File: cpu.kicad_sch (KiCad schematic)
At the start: 33 parts, among them IC12 DS2401+, IC13 ARM250, IC20 74HC138, IC27 74AC32, IC8 74HCT14, X4 72.0MHz, X5 25.175MHz

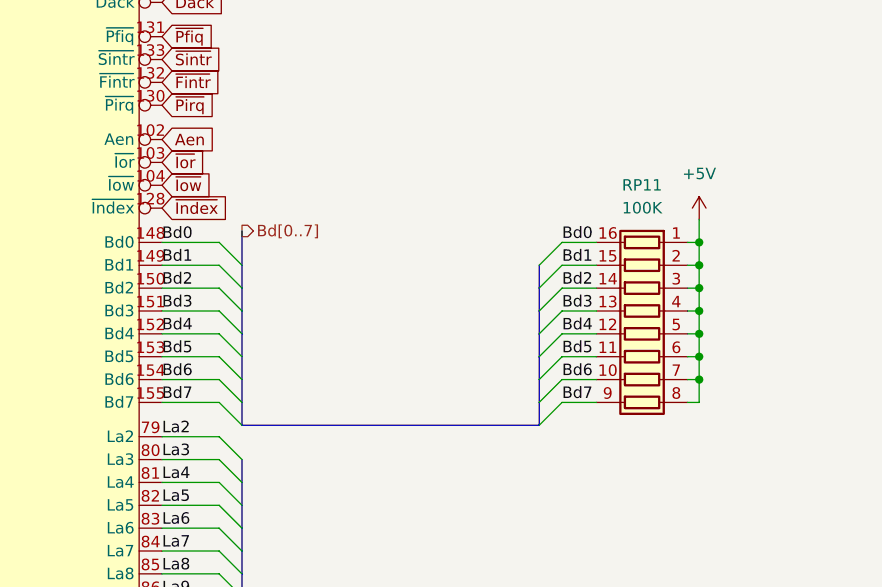
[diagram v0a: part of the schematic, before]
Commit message: fix rp11
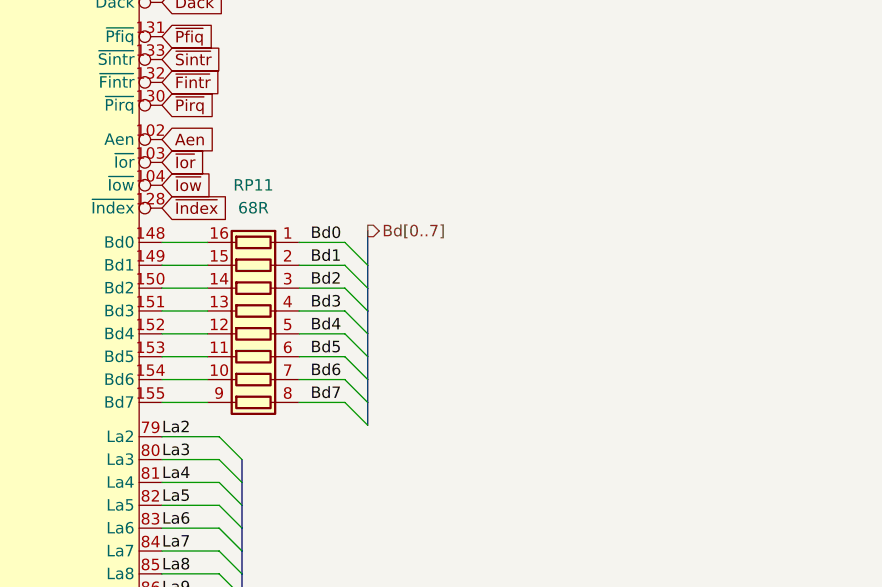
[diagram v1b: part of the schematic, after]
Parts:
- RP11: value 100K -> 68R
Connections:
- net +5V: no longer RP11.1 (R1.1), RP11.2 (R2.1), RP11.3 (R3.1), RP11.4 (R4.1), RP11.5 (R5.1), RP11.6 (R6.1), RP11.7 (R7.1), RP11.8 (R8.1)
- net Bd0: now also RP11.1 (R1.1); no longer IC13.148 (Bd0), RP11.16 (R1.2)
- net Bd1: now also RP11.2 (R2.1); no longer IC13.149 (Bd1), RP11.15 (R2.2)
- net Bd2: now also RP11.3 (R3.1); no longer IC13.150 (Bd2), RP11.14 (R3.2)
- net Bd3: now also RP11.4 (R4.1); no longer IC13.151 (Bd3), RP11.13 (R4.2)
- net Bd4: now also RP11.5 (R5.1); no longer IC13.152 (Bd4), RP11.12 (R5.2)
- net Bd5: now also RP11.6 (R6.1); no longer IC13.153 (Bd5), RP11.11 (R6.2)
- net Bd6: now also RP11.7 (R7.1); no longer IC13.154 (Bd6), RP11.10 (R7.2)
- net Bd7: now also RP11.8 (R8.1); no longer IC13.155 (Bd7), RP11.9 (R8.2)
- new net: IC13.154 (Bd6), RP11.10 (R7.2)
- new net: IC13.153 (Bd5), RP11.11 (R6.2)
- new net: IC13.152 (Bd4), RP11.12 (R5.2)
- new net: IC13.151 (Bd3), RP11.13 (R4.2)
- new net: IC13.150 (Bd2), RP11.14 (R3.2)
- new net: IC13.149 (Bd1), RP11.15 (R2.2)
- new net: IC13.148 (Bd0), RP11.16 (R1.2)
- new net: IC13.155 (Bd7), RP11.9 (R8.2)
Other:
- moved on the sheet: RP11

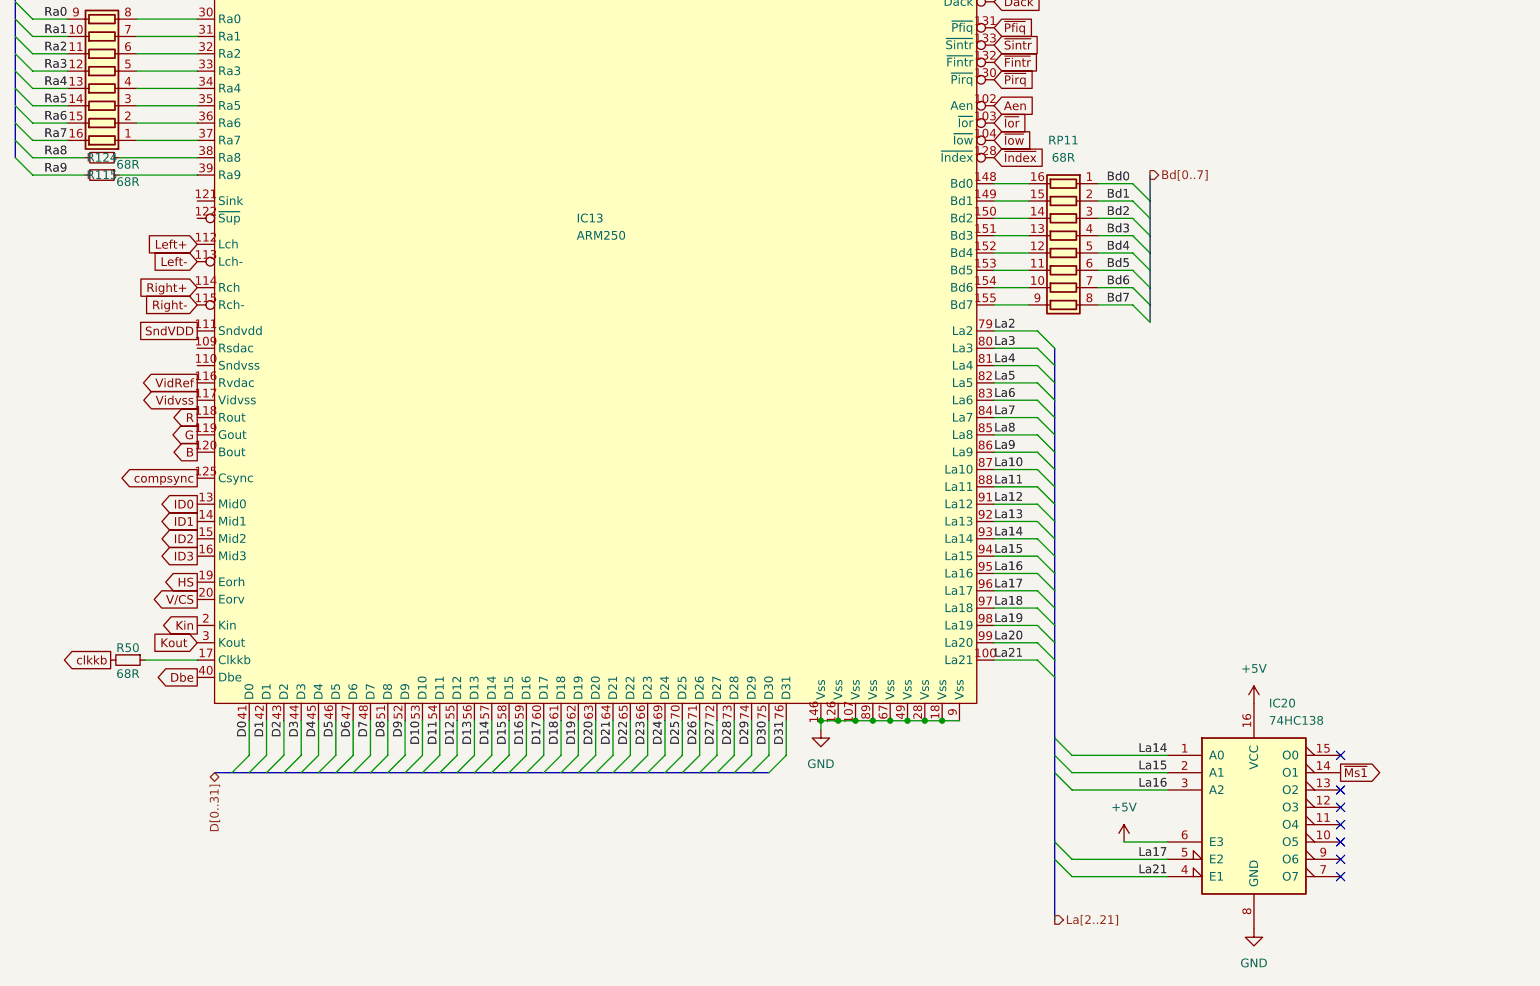
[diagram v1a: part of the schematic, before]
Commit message: more traces
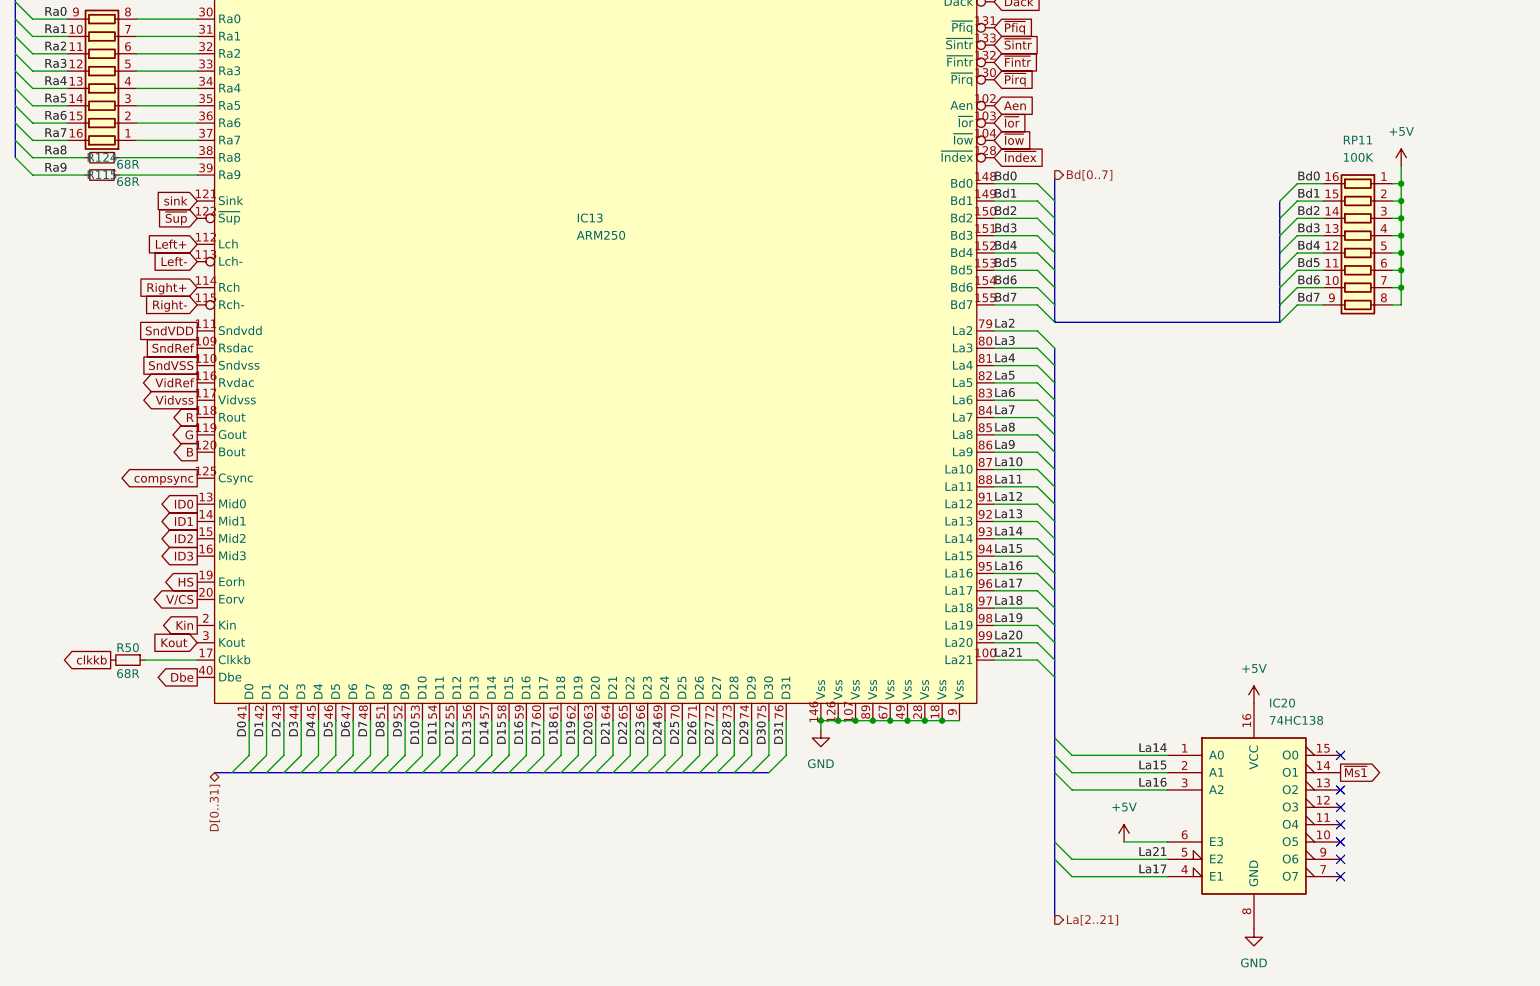
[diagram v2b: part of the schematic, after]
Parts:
- RP11: value 68R -> 100K
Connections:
- net +5V: now also RP11.1 (R1.1), RP11.2 (R2.1), RP11.3 (R3.1), RP11.4 (R4.1), RP11.5 (R5.1), RP11.6 (R6.1), RP11.7 (R7.1), RP11.8 (R8.1)
- net Bd0: now also IC13.148 (Bd0), RP11.16 (R1.2); no longer RP11.1 (R1.1)
- net Bd1: now also IC13.149 (Bd1), RP11.15 (R2.2); no longer RP11.2 (R2.1)
- net Bd2: now also IC13.150 (Bd2), RP11.14 (R3.2); no longer RP11.3 (R3.1)
- net Bd3: now also IC13.151 (Bd3), RP11.13 (R4.2); no longer RP11.4 (R4.1)
- net Bd4: now also IC13.152 (Bd4), RP11.12 (R5.2); no longer RP11.5 (R5.1)
- net Bd5: now also IC13.153 (Bd5), RP11.11 (R6.2); no longer RP11.6 (R6.1)
- net Bd6: now also IC13.154 (Bd6), RP11.10 (R7.2); no longer RP11.7 (R7.1)
- net Bd7: now also IC13.155 (Bd7), RP11.9 (R8.2); no longer RP11.8 (R8.1)
- net La17: now also IC20.4 (E1); no longer IC20.5 (E2)
- net La21: now also IC20.5 (E2); no longer IC20.4 (E1)
- net SndRef: now reaches IC13.109 (Rsdac)
- net SndVSS: now reaches IC13.110 (Sndvss)
- net sink: now reaches IC13.121 (Sink)
- net ~{Sup}: now reaches IC13.122 (~{Sup})
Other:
- moved on the sheet: RP11
